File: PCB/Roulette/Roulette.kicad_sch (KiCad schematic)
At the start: 275 parts, among them J1 USB-PROG, J2 Shelly, J3 53261-0271, J3 Conn_01x03, J4 Conn_01x02, J6 GT-USB-7082C, Q1 PMF170XP,115, Q4 CJ2301, SW1 SW_Push, U2 ESP32-S3-MINI-1, U2 ME6211C33M5G-N, U5 TP4054

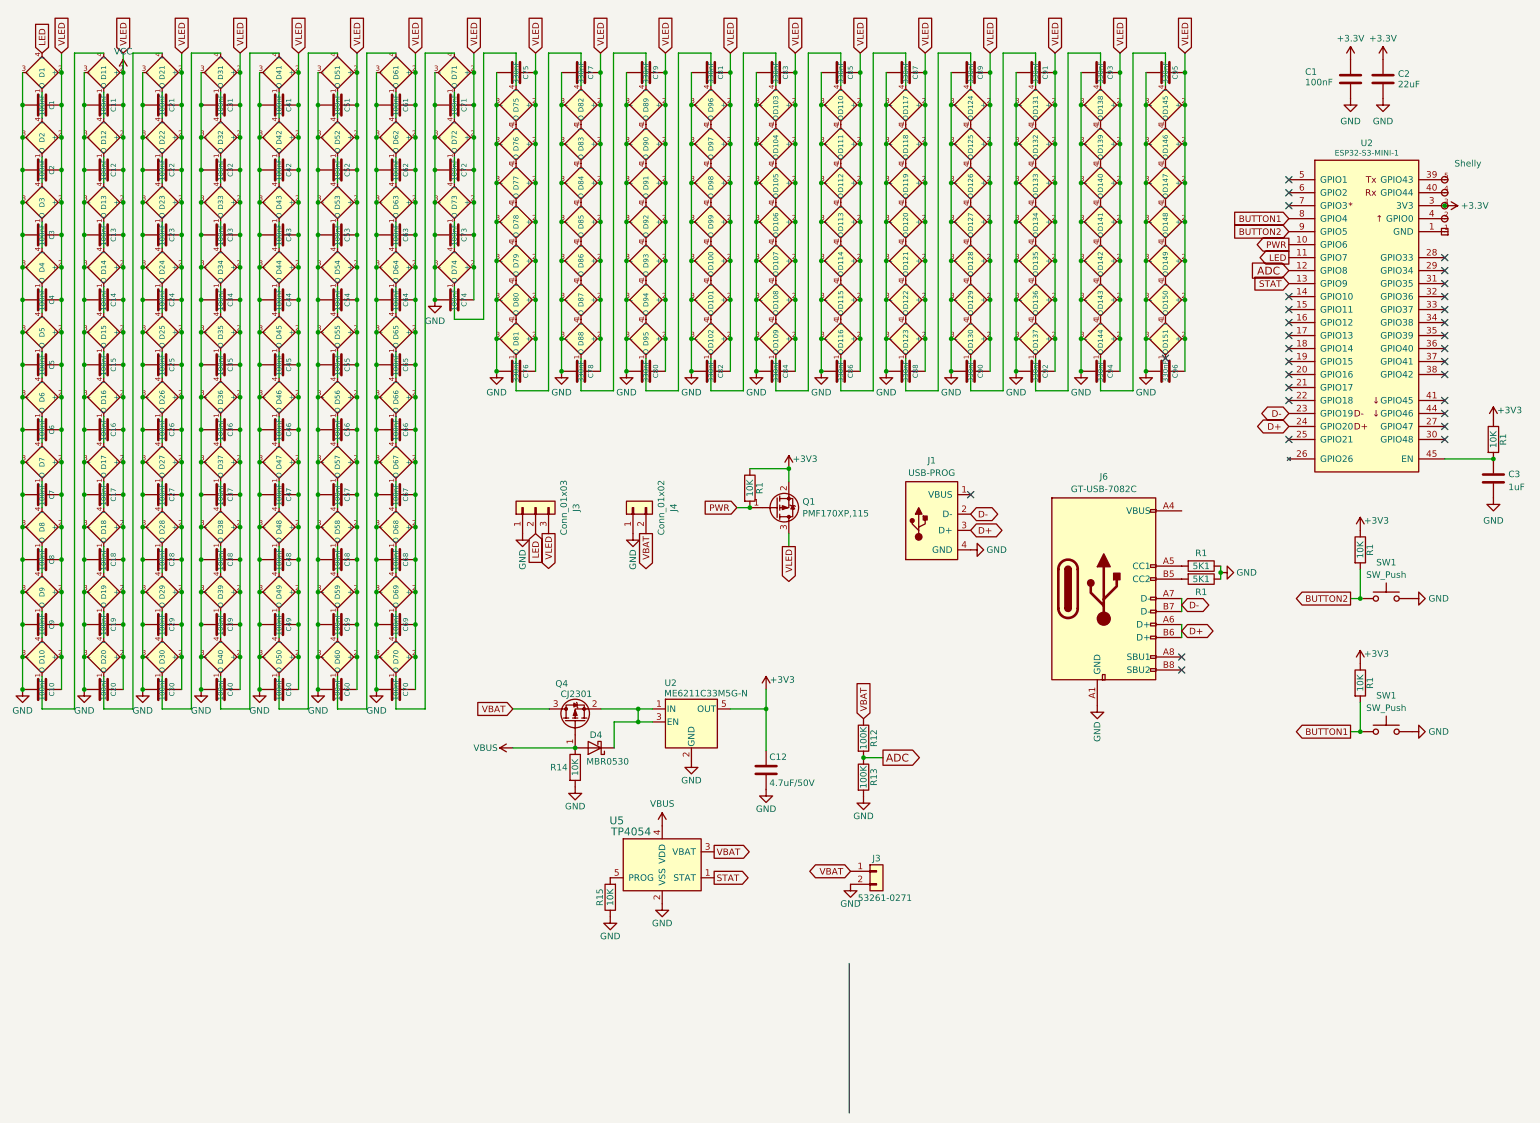
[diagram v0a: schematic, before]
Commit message: Rechargable board
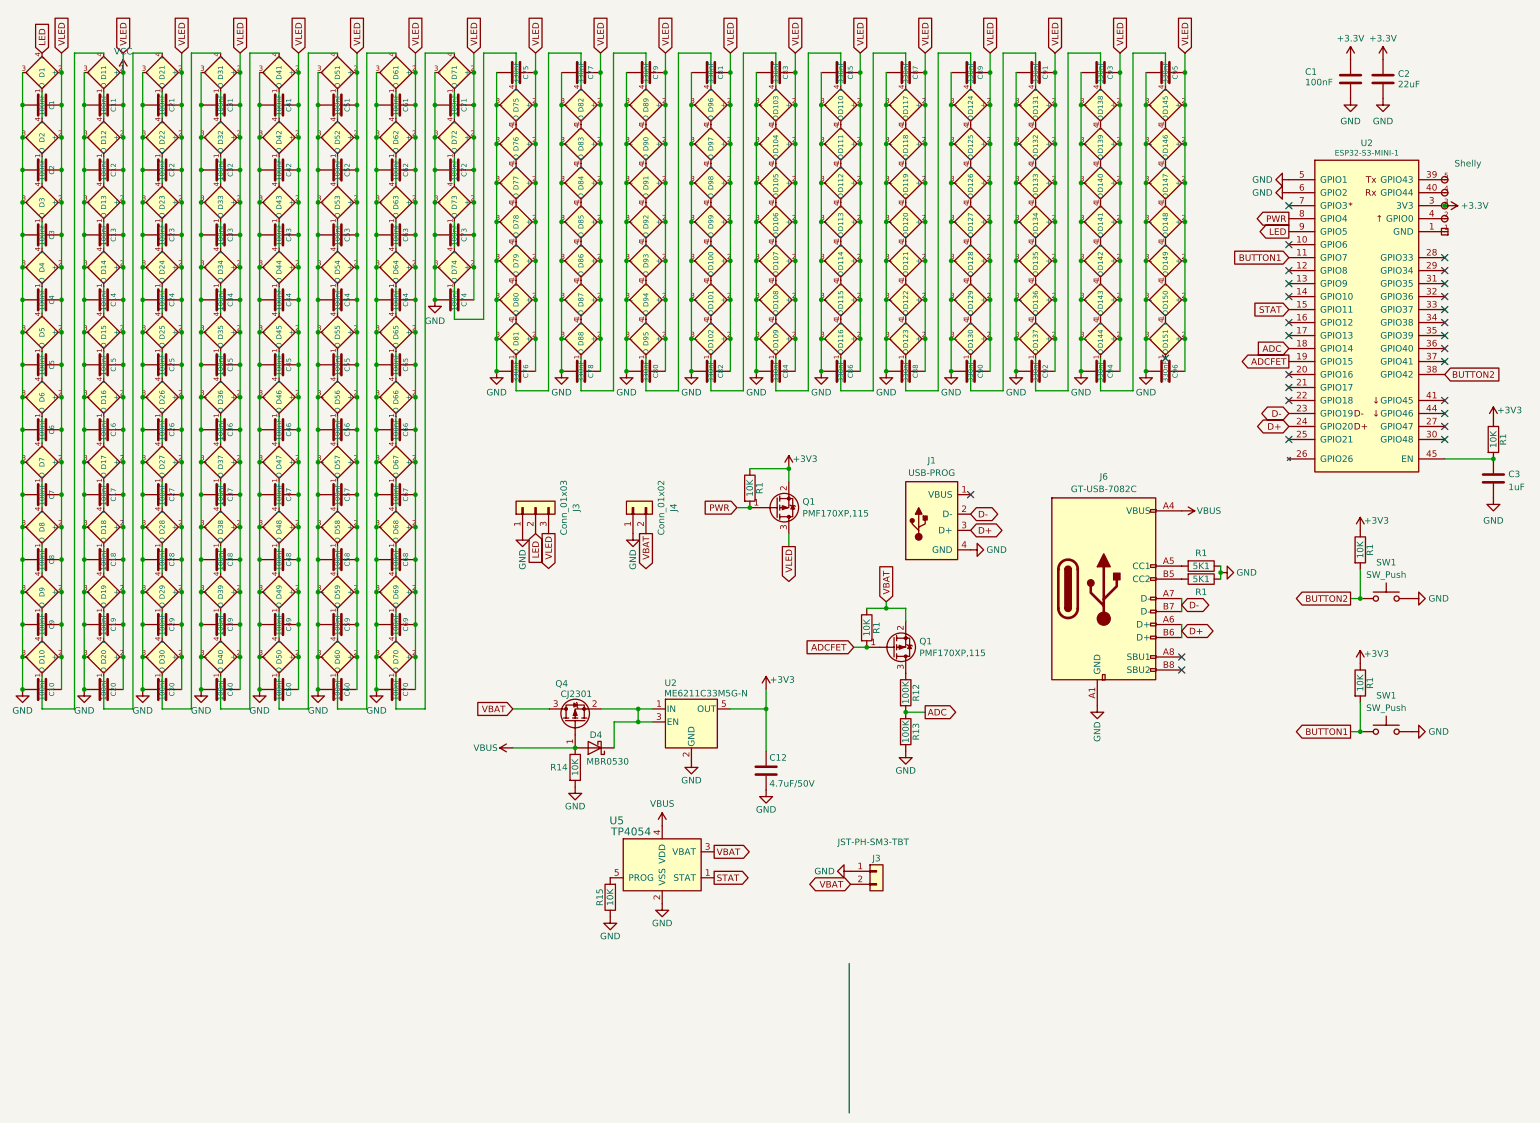
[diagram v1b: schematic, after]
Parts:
- added Q1: PMF170XP,115, RevK:SOT-323_SC-70, symbol Device:Q_PMOS_GSD
- added R1: 10K, RevK:R_0402, symbol Device:R
- J3: value 53261-0271 -> JST-PH-SM3-TBT; footprint Connector_Molex:Molex_PicoBlade_53261-0271_1x02-1MP_P1.25mm_Horizontal -> Connector_JST:JST_PH_B2B-PH-SM4-TB_1x02-1MP_P2.00mm_Vertical; LCSC Part # C189700 -> C265003
- J6: LCSC Part # C3001289 -> C3001291
- Q4: LCSC Part # (none) -> C5224170
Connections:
- net ADC: now also U2.18 (GPIO14); no longer U2.12 (GPIO8)
- net BUTTON1: now also U2.11 (GPIO7); no longer U2.8 (GPIO4)
- net BUTTON2: now also U2.38 (GPIO42); no longer U2.9 (GPIO5)
- net GND: now also J3.1 (Pin_1), J6.A12 (GND), J6.B1 (GND), J6.B12 (GND), U2.5 (GPIO1), U2.6 (GPIO2); no longer J3.2 (Pin_2)
- net LED: now also U2.9 (GPIO5); no longer U2.11 (GPIO7)
- net PWR: now also U2.8 (GPIO4); no longer U2.10 (GPIO6)
- net STAT: now also U2.15 (GPIO11); no longer U2.13 (GPIO9)
- net VBAT: now also J3.2 (Pin_2), Q1.2 (S), R1.1; no longer J3.1 (Pin_1), R12.1
- net VBUS: now also J6.A4 (VBUS), J6.A9 (VBUS), J6.B4 (VBUS), J6.B9 (VBUS)
- net ADCFET: now reaches U2.19 (GPIO15)
- net ADCFET: now also Q1.1 (G), R1.2
- new net: Q1.3 (D), R12.1
- no-connect marks 31 -> 28
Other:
- moved on the sheet: R12, R13
